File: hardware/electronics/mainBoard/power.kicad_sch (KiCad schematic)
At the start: 9 parts

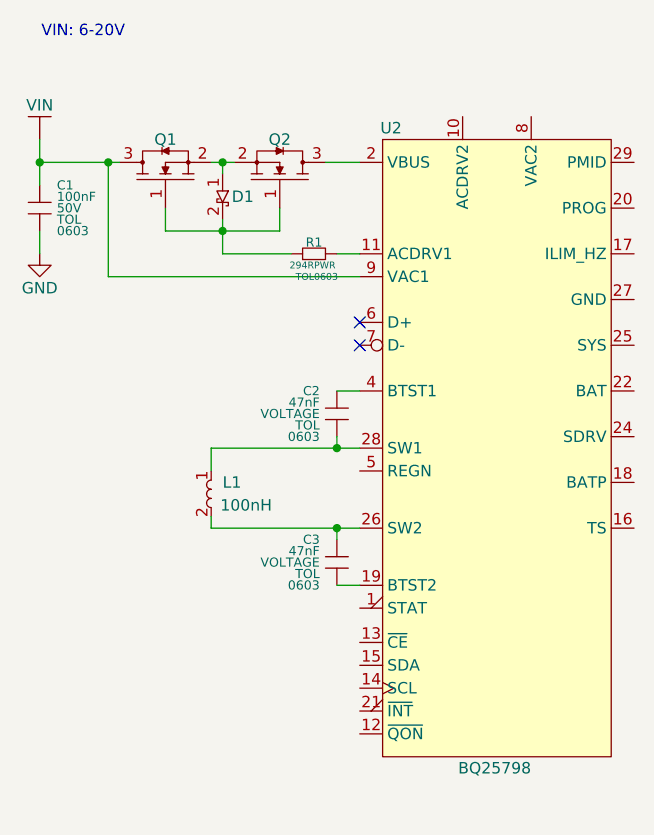
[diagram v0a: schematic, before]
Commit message: batt charger stuff
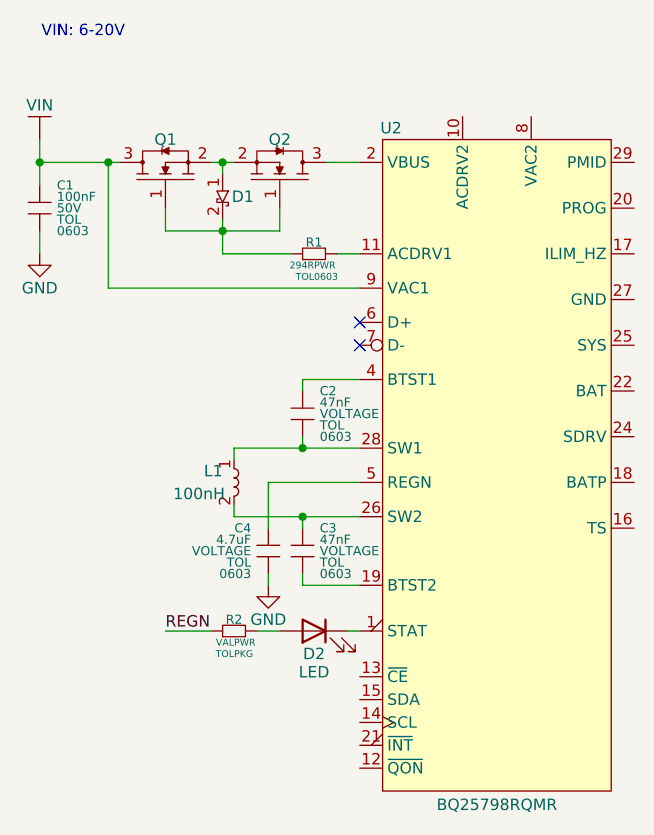
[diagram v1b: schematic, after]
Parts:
- added C4: 4.7uF, symbol DSE-Passives:C
- added D2: LED, symbol Device:LED
- added R2: VAL, symbol DSE-Passives:R_horizontal
- U2: value ~ -> BQ25798RQMR
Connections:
- net GND: now also C4.2
- net at U2.1 (STAT): now also D2.1 (K)
- net at U2.5 (REGN): now also C4.1
- new net: D2.2 (A), R2.2
- new net REGN: R2.1
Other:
- moved on the sheet: C2, C3, U2
